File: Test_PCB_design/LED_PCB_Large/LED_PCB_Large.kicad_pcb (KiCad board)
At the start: 2 copper layers, 88.7 x 182.4 mm, 113 parts, among them J1 AS150UPB 2+4, Q1 BUK9Y107-80EX, Q10 BUK9Y107-80EX, Q11 BUK9Y107-80EX, Q12 BUK9Y107-80EX, Q2 BUK9Y107-80EX, Q3 BUK9Y107-80EX, Q4 BUK9Y107-80EX, Q5 BUK9Y107-80EX, Q6 BUK9Y107-80EX, Q7 BUK9Y107-80EX, Q8 BUK9Y107-80EX, Q9 BUK9Y107-80EX, U1 MAX20078ATE_V_T, U2 MAX20078ATE_V_T, U3 MAX20078ATE_V_T, U4 MAX20078ATE_V_T, U5 MAX20078ATE_V_T, U6 MAX20078ATE_V_T

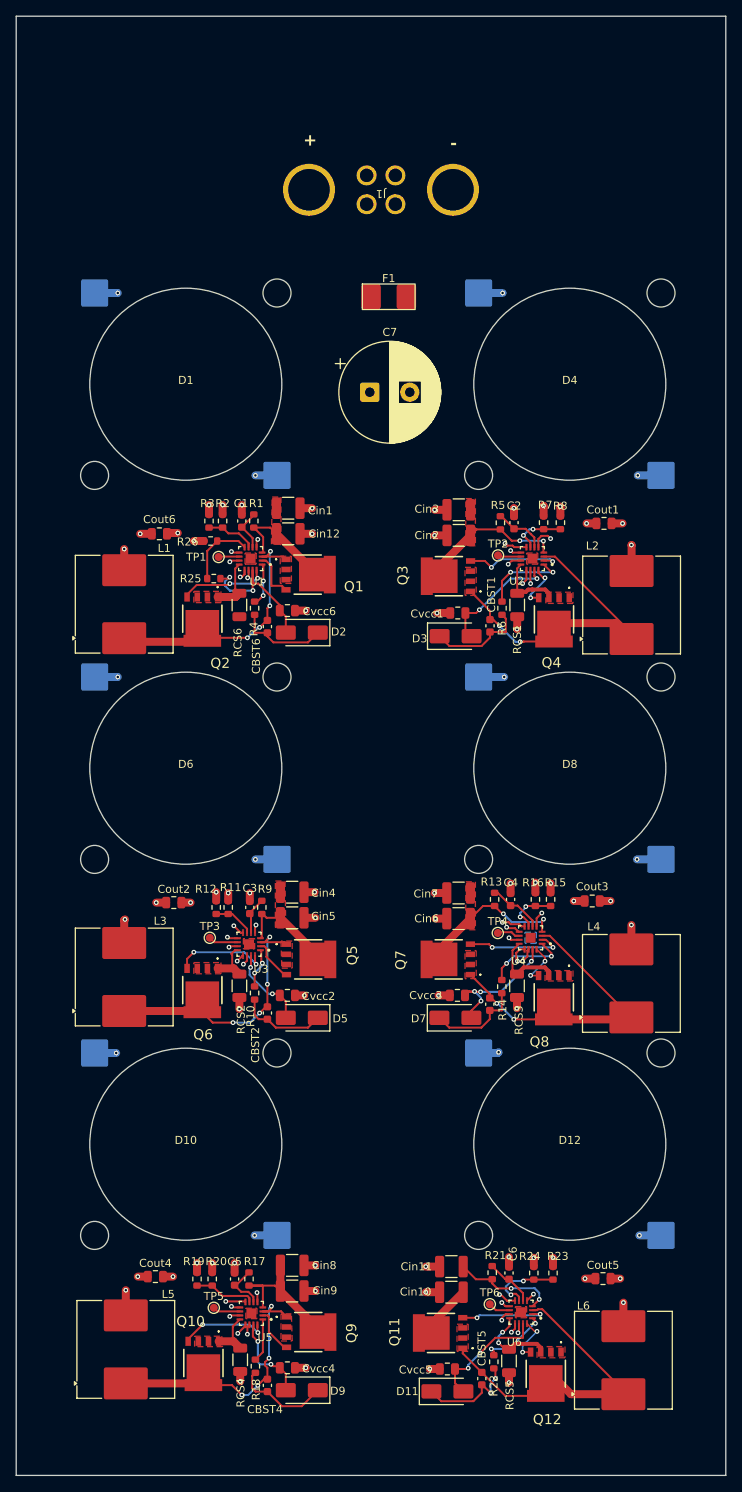
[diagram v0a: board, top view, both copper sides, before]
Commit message: updated everything just need to check electrical traces to make sure they work.
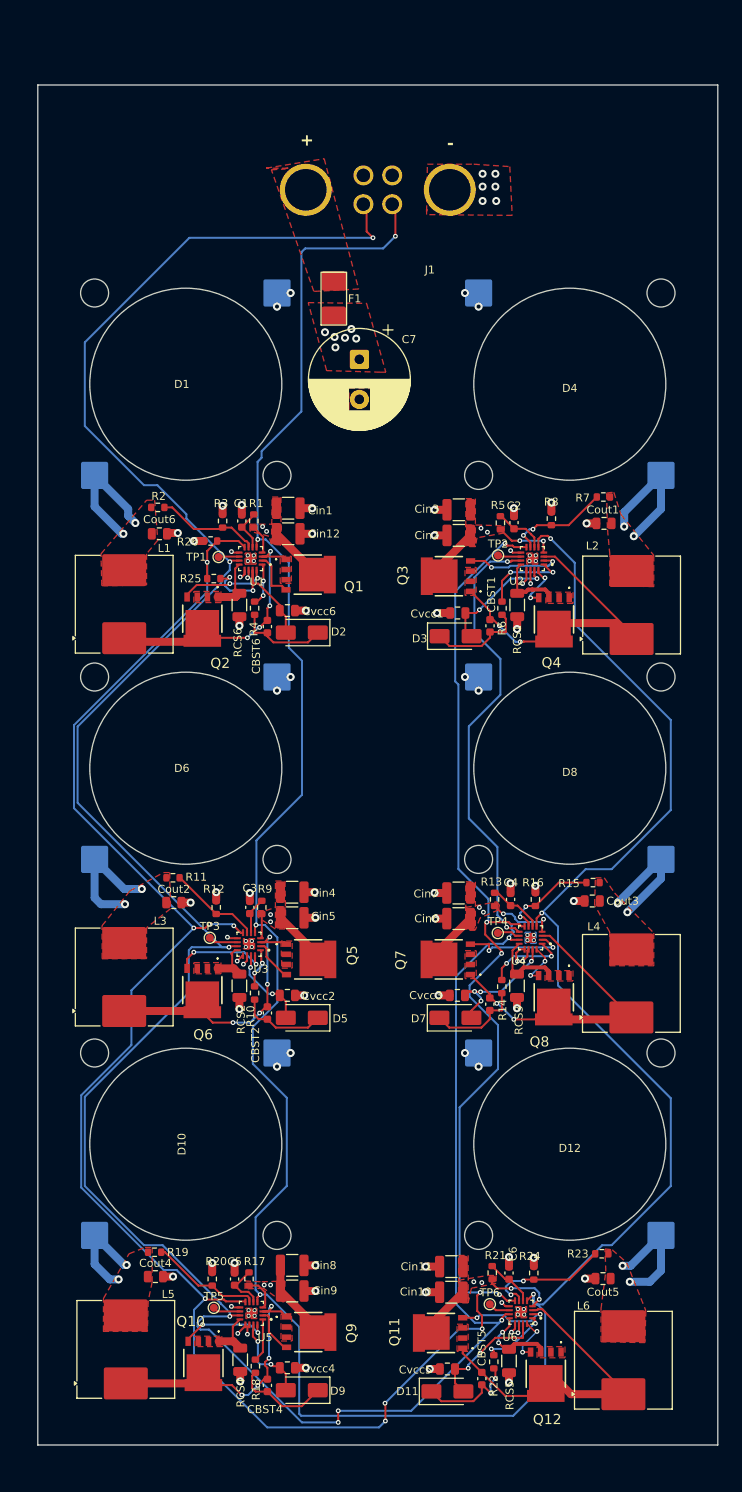
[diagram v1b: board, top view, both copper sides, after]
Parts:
- moved R2 8.28 mm to (96.0, 46.4), turned to 0 degrees
- moved R7 8.13 mm to (151.7, 45.1), turned to 180 degrees
- moved R11 7.83 mm to (97.9, 92.7), turned to 0 degrees
- moved F1 6.87 mm to (118.0, 20.3), turned to 90 degrees
- moved R23 6.56 mm to (151.5, 139.7), turned to 180 degrees
- moved R19 6.27 mm to (95.6, 139.5), turned to 0 degrees
- moved R15 5.70 mm to (150.4, 93.3), turned to 180 degrees
- moved C7 4.30 mm to (121.2, 27.9), turned to -90 degrees
- moved R3 1.70 mm to (104.1, 48.1)
- moved R8 1.23 mm to (145.2, 47.8)
- moved J1 0.40 mm to (123.5, 6.70)
- turned Cout5 to 180 degrees
- turned D1 to 90 degrees
- turned D10 to 90 degrees
- turned D12 to 180 degrees
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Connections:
- Cout1 pad 1: /LED+ -> /LED2+
- Cout2 pad 1: /LED+ -> /LED3+
- Cout3 pad 1: /LED+ -> /LED4+
- Cout4 pad 1: /LED+ -> /LED5+
- Cout5 pad 1: /LED+ -> /LED6+
- Cout6 pad 1: /LED+ -> /LED1+
- D1 pad 2: /LED+ -> /LED1+
- D10 pad 2: /LED+ -> /LED5+
- D12 pad 2: /LED+ -> /LED6+
- D4 pad 2: /LED+ -> /LED2+
- D6 pad 2: /LED+ -> /LED3+
- D8 pad 2: /LED+ -> /LED4+
- L1 pad 2: /LED+ -> /LED1+
- L2 pad 2: /LED+ -> /LED2+
- L3 pad 2: /LED+ -> /LED3+
- L4 pad 2: /LED+ -> /LED4+
- L5 pad 2: /LED+ -> /LED5+
- L6 pad 2: /LED+ -> /LED6+
- R11 pad 1: /LED+ -> /LED3+
- R15 pad 1: /LED+ -> /LED4+
- R19 pad 1: /LED+ -> /LED5+
- R2 pad 1: /LED+ -> /LED1+
- R23 pad 1: /LED+ -> /LED6+
- R7 pad 1: /LED+ -> /LED2+
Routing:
- net /FAULT: track 8.25 -> 386.0 mm, vias 6 -> 9
- net /PWM: track 9.17 -> 359.0 mm, vias 6 -> 7
- net /REF_1V2: track 21.1 -> 317.1 mm, vias 5 -> 13
- net /LED+: track 50.6 -> 0.00 mm, vias 24 -> 0
- net +48V_FUSED: track 101.8 -> 80.7 mm, vias 6 -> 24
- net /LED2+: track 0.00 -> 17.3 mm, vias 0 -> 2
- net /LED1+: track 0.00 -> 17.0 mm, vias 0 -> 2
- net /LED3+: track 0.00 -> 16.4 mm, vias 0 -> 2
- net /LED4+: track 0.00 -> 16.1 mm, vias 0 -> 2
- net /LED6+: track 0.00 -> 15.3 mm, vias 0 -> 2
- net /LED5+: track 0.00 -> 12.9 mm, vias 0 -> 2
- net Net-(U1-OUT): track 6.26 -> 13.0 mm
- net Net-(U6-OUT): track 9.29 -> 15.9 mm
- net Net-(U3-OUT): track 5.11 -> 11.6 mm
- net Net-(U2-OUT): track 6.77 -> 13.0 mm
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- added copper zone on In2.Cu, net +48V_FUSED
- added copper zone on F.Cu, net /LED1+
- added copper zone on F.Cu, net /LED2+
- added copper zone on F.Cu, net /LED3+
- added copper zone on F.Cu, net /LED4+
- added copper zone on F.Cu, net /LED5+
- added copper zone on F.Cu, net /LED6+
- added copper zone on In1.Cu, net GND
- added copper zone on F.Cu, net Net-(J1-+48V)
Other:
- board size 88.7 x 182.4 mm -> 85 x 170 mm
- copper layers 2 -> 4
